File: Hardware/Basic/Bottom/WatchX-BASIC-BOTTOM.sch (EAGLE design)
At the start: 31 parts, among them U1 AD5242-SO16

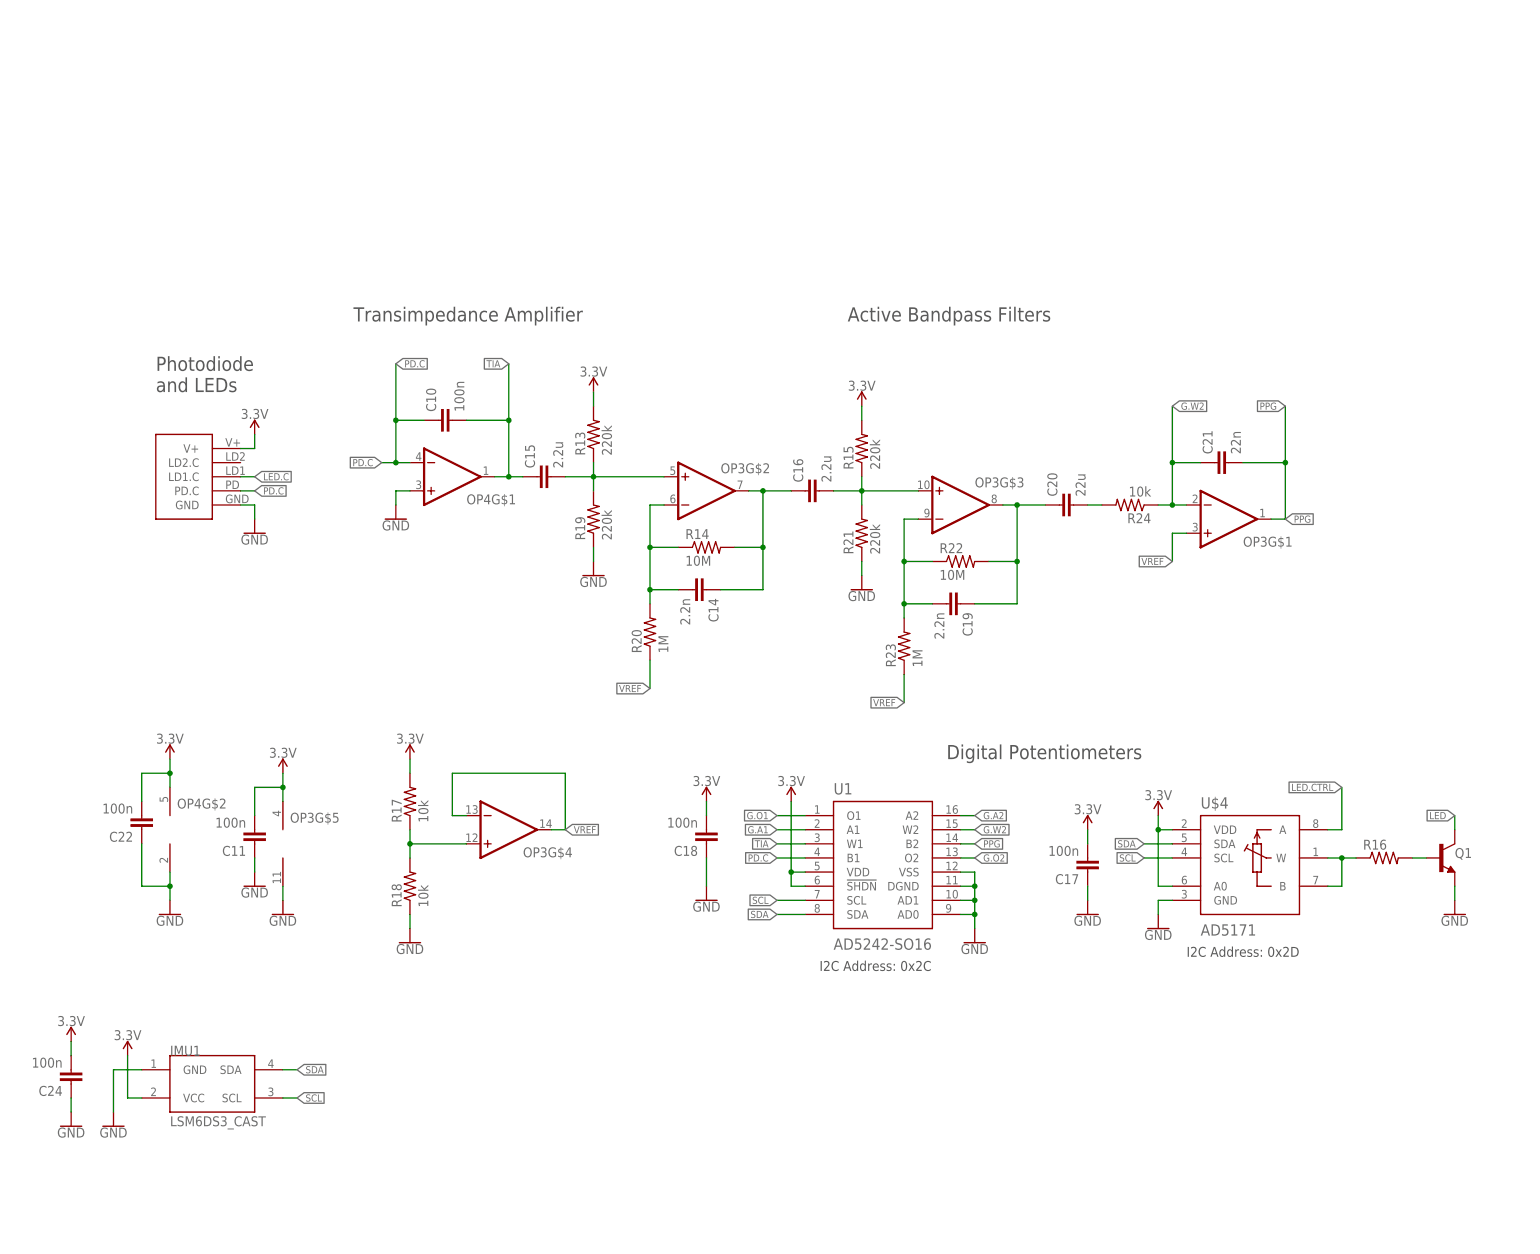
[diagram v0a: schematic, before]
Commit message: changes up to take 003
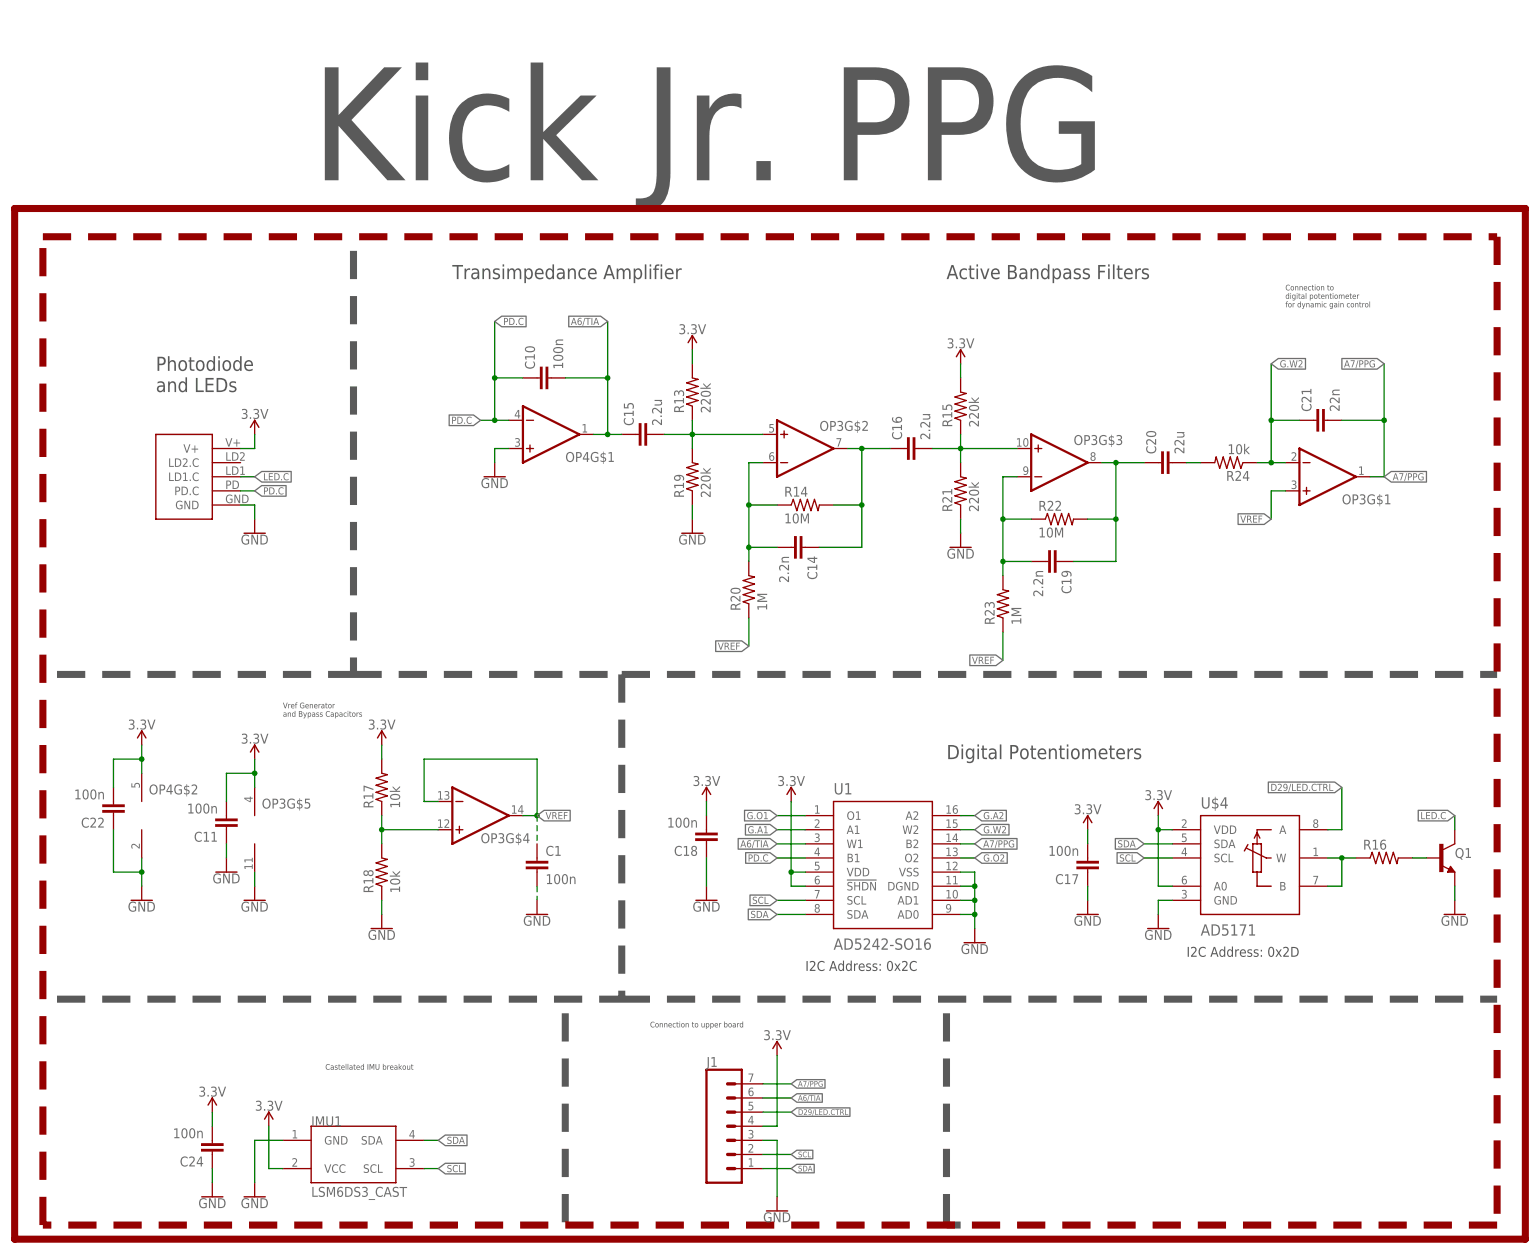
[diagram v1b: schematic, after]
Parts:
- added C1: 100n, LinnesLab-Passives:CAPACITOR0603
- added J1: (no value), LinnesLab-Connectors:CONN_07-1.27MM
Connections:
- removed net LED: Q1.C
- removed net LED.CTRL: U$4.A
- removed net PPG: C21.2, OP3G$1.OUT, U1.B2
- removed net TIA: C10.2, C15.1, OP4G$1.OUT, U1.W1
- new net A6/TIA: C10.2, C15.1, J1.6, OP4G$1.OUT, U1.W1
- new net A7/PPG: C21.2, J1.7, OP3G$1.OUT, U1.B2
- new net D29/LED.CTRL: J1.5, U$4.A
- net 3.3V: now also J1.4
- net GND: now also C1.2, J1.3
- net LED.C: now also Q1.C
- net SCL: now also J1.2
- net SDA: now also J1.1
- net VREF: now also C1.1
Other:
- note added: "Castellated IMU breakout"
- note added: "Connection to digital potentiometer for dynamic gain control"
- note added: "Connection to upper board"
- note added: "Kick Jr. PPG"
- note added: "Vref Generator and Bypass Capacitors"
- moved on the sheet: C10, C11, C14, C15, C16, C19, C20, C21, C22, C24, IMU1, OP3G$1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
